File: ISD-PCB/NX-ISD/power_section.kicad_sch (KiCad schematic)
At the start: 34 parts, among them J2 UJ20-C-H-G-SMT-1-P16-TR, P1 S2B-PH-SM4-TB, Q2 AO3401A, Q3 BC847W, U13 RT9193-18GB, U15 USBLC6-2P6, U2 TLV62568DBV, U8 BQ25170DSGR, U9 RT9193-28GB

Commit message: Added 3D-Renders to README
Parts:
- J2: footprint NX-AW-footprints:SAMESKY_UJ20-C-H-G-SMT-1-P16-TR -> Global Footprints:SAMESKY_UJ20-C-H-G-SMT-1-P16-TR
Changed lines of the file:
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@@
 			)
 		)
-		(property "Footprint" "NX-AW-footprints:SAMESKY_UJ20-C-H-G-SMT-1-P16-TR"
+		(property "Footprint" "Global Footprints:SAMESKY_UJ20-C-H-G-SMT-1-P16-TR"
 			(at 30.48 55.88 0)
 			(hide yes)

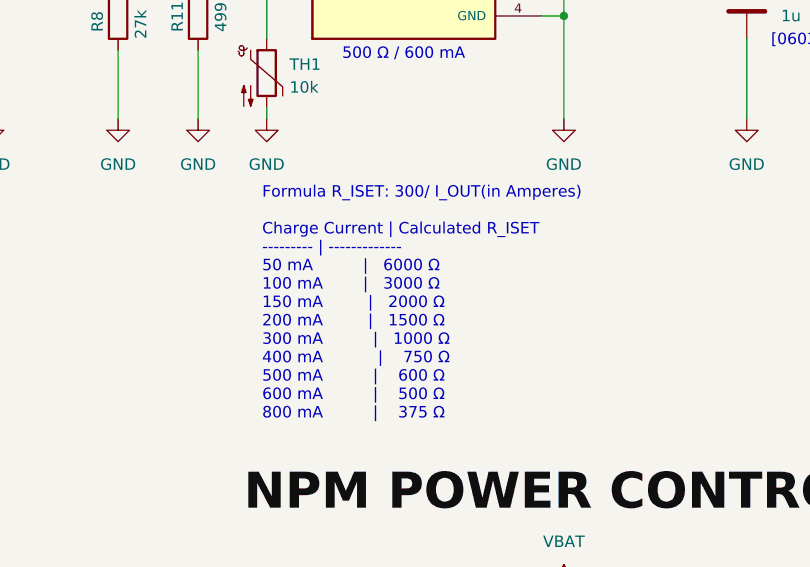
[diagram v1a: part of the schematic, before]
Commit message: v1p3 production ready
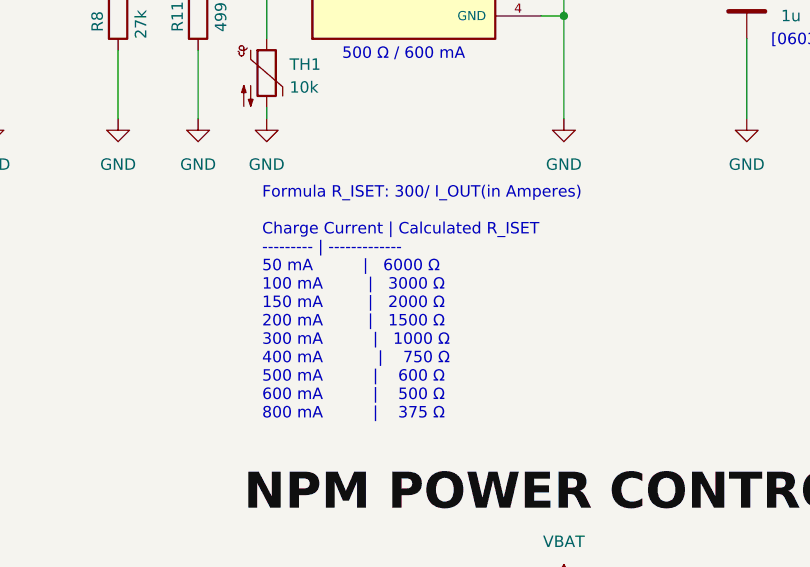
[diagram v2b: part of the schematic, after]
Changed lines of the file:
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@@
 		)
 	)
-	(text "Formula R_ISET: 300/ I_OUT(in Amperes)\n\nCharge Current | Calculated R_ISET\n--------- | -------------\n50 mA	      |   6000 Ω\n100 mA        |   3000 Ω\n150 mA		 |   2000 Ω\n200 mA		 |   1500 Ω\n300 mA	      |   1000 Ω\n400 mA 	      |    750 Ω\n500 mA	      |    600 Ω\n600 mA	      |    500 Ω\n800 mA	      |    375 Ω"
+	(text "Formula R_ISET: 300/ I_OUT(in Amperes)\n\nCharge Current | Calculated R_ISET\n--------- | -------------\n50 mA	      |   6000 Ω\n100 mA         |   3000 Ω\n150 mA		 |   2000 Ω\n200 mA		 |   1500 Ω\n300 mA	      |   1000 Ω\n400 mA 	      |    750 Ω\n500 mA	      |    600 Ω\n600 mA	      |    500 Ω\n800 mA	      |    375 Ω"
 		(exclude_from_sim no)
 		(at 206.502 96.774 0)
